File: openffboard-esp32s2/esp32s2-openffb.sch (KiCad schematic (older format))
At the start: 31 parts, among them J2 Debug, J3 CAN_Connector, J4 Motor Driver, SW1 SW_Push, SW2 SW_Push, U1 AMS1117-3.3, U3 TJA1051T-3, U5 ESP32-S2-SOLO

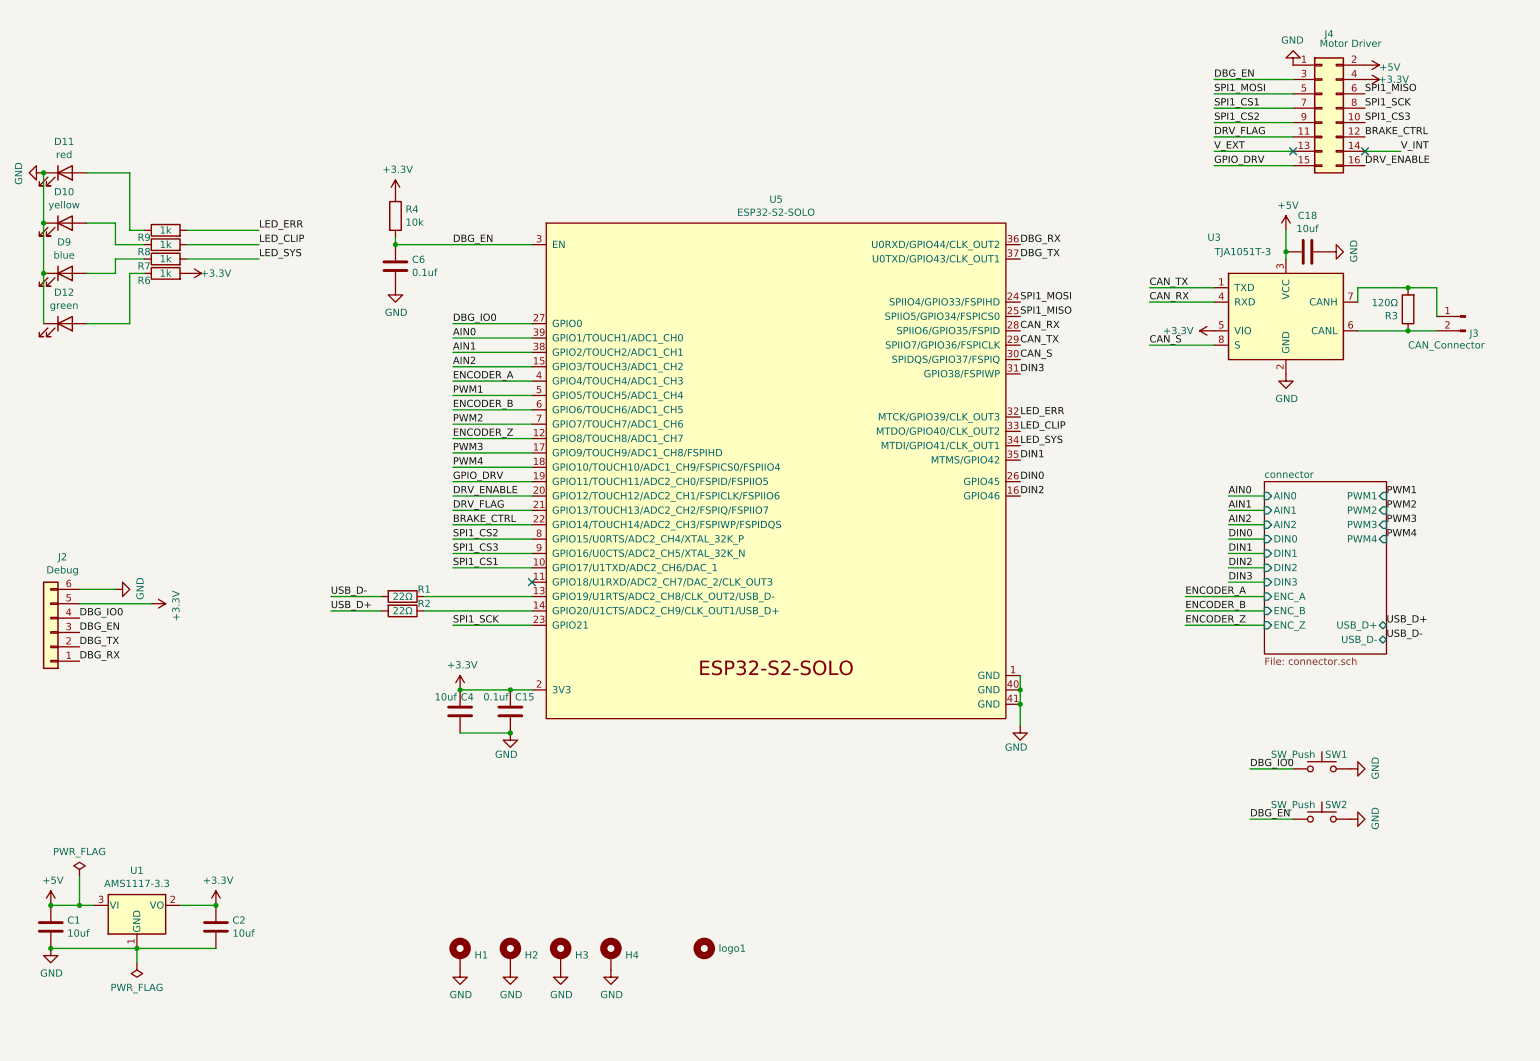
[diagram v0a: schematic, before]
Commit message: v1.1
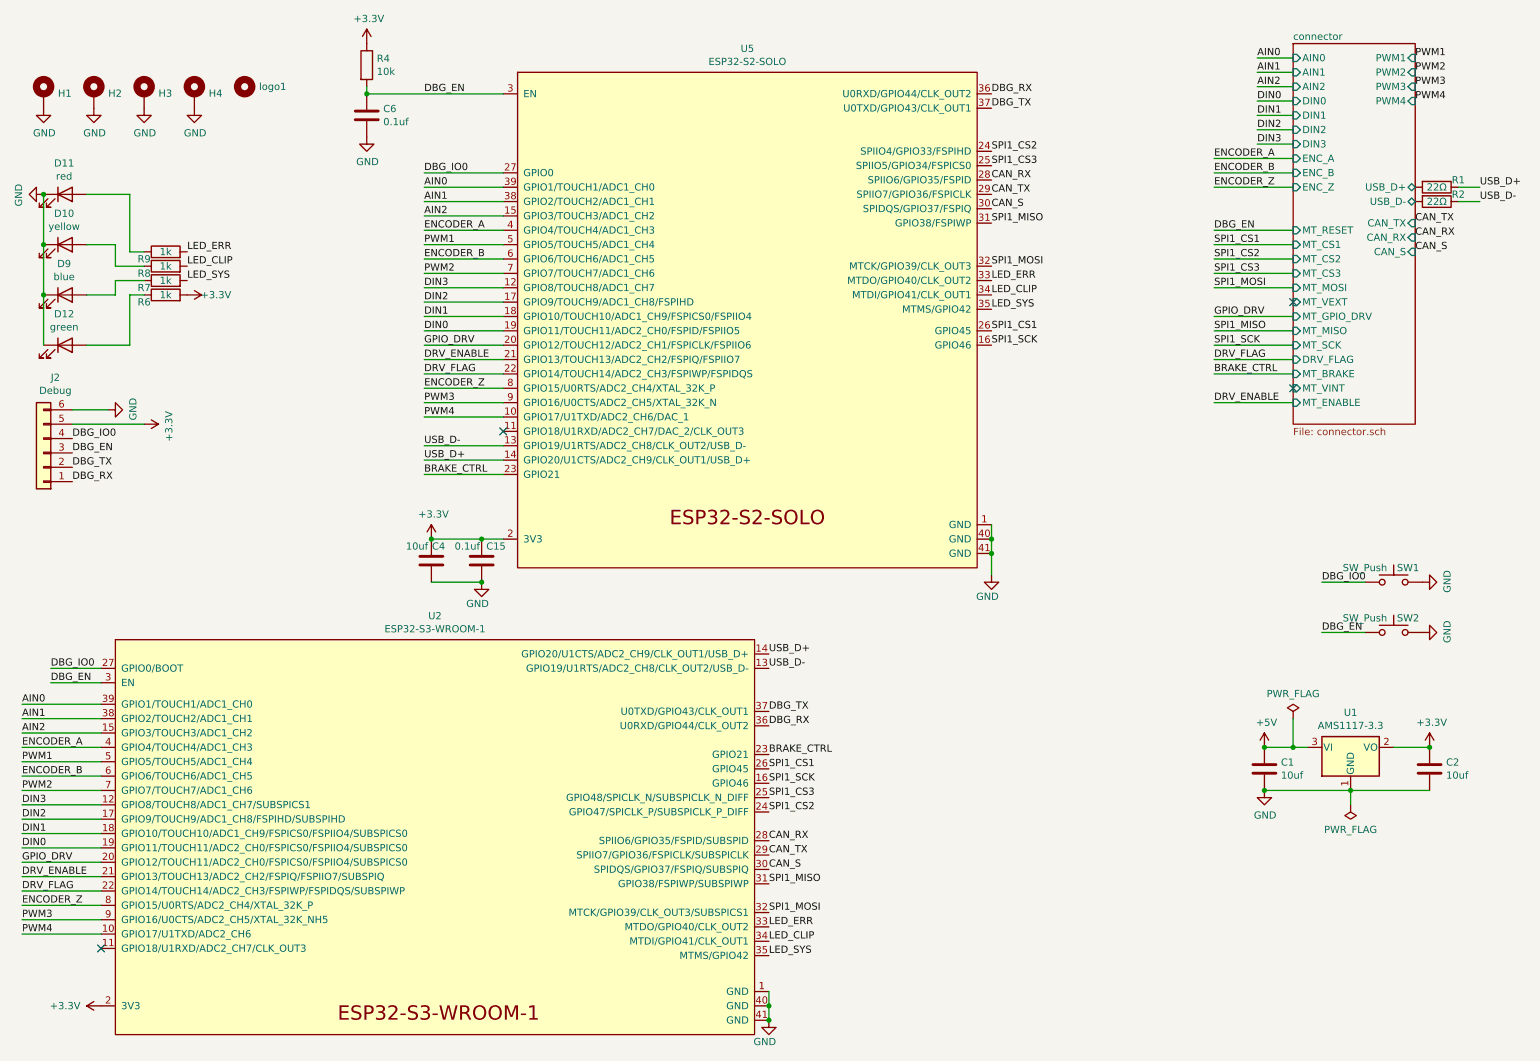
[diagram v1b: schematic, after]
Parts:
- removed C18: 10uf, Capacitor_SMD:C_0603_1608Metric, symbol Device:C
- removed J3: CAN_Connector, Connector_PinHeader_2.54mm:PinHeader_1x02_P2.54mm_Vertical, symbol Connector:Conn_01x02_Male
- removed J4: Motor Driver, Connector_PinHeader_2.54mm:PinHeader_2x08_P2.54mm_Vertical, symbol Connector_Generic:Conn_02x08_Odd_Even
- removed R3: 120Ω, Resistor_SMD:R_0603_1608Metric, symbol Device:R
- removed U3: TJA1051T-3, Package_SO:SOIC-8_3.9x4.9mm_P1.27mm, symbol Interface_CAN_LIN:TJA1051T-3
- added U2: ESP32-S3-WROOM-1, Espressif:ESP32-S3-WROOM-1, symbol Espressif:ESP32-S3-WROOM-1
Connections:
- net +3V3: now also U2.2 (3V3)
- net AIN0: now also U2.39 (GPIO1/TOUCH1/ADC1_CH0)
- net AIN1: now also U2.38 (GPIO2/TOUCH2/ADC1_CH1)
- net AIN2: now also U2.15 (GPIO3/TOUCH3/ADC1_CH2)
- net BRAKE_CTRL: now also U5.23 (GPIO21), U2.23 (GPIO21); no longer U5.22 (GPIO14/TOUCH14/ADC2_CH3/FSPIWP/FSPIDQS)
- net CAN_RX: now also U2.28 (SPIIO6/GPIO35/FSPID/SUBSPID)
- net CAN_S: now also U2.30 (SPIDQS/GPIO37/FSPIQ/SUBSPIQ)
- net CAN_TX: now also U2.29 (SPIIO7/GPIO36/FSPICLK/SUBSPICLK)
- net DBG_EN: now also U2.3 (EN)
- net DBG_IO0: now also U2.27 (GPIO0/BOOT)
- net DBG_RX: now also U2.36 (U0RXD/GPIO44/CLK_OUT2)
- net DBG_TX: now also U2.37 (U0TXD/GPIO43/CLK_OUT1)
- net DIN0: now also U5.19 (GPIO11/TOUCH11/ADC2_CH0/FSPID/FSPIIO5), U2.19 (GPIO11/TOUCH11/ADC2_CH0/FSPICS0/FSPIIO4/SUBSPICS0); no longer U5.26 (GPIO45)
- net DIN1: now also U5.18 (GPIO10/TOUCH10/ADC1_CH9/FSPICS0/FSPIIO4), U2.18 (GPIO10/TOUCH10/ADC1_CH9/FSPICS0/FSPIIO4/SUBSPICS0); no longer U5.35 (MTMS/GPIO42)
- net DIN2: now also U5.17 (GPIO9/TOUCH9/ADC1_CH8/FSPIHD), U2.17 (GPIO9/TOUCH9/ADC1_CH8/FSPIHD/SUBSPIHD); no longer U5.16 (GPIO46)
- net DIN3: now also U5.12 (GPIO8/TOUCH8/ADC1_CH7), U2.12 (GPIO8/TOUCH8/ADC1_CH7/SUBSPICS1); no longer U5.31 (GPIO38/FSPIWP)
- net DRV_ENABLE: now also U5.21 (GPIO13/TOUCH13/ADC2_CH2/FSPIQ/FSPIIO7), U2.21 (GPIO13/TOUCH13/ADC2_CH2/FSPIQ/FSPIIO7/SUBSPIQ); no longer U5.20 (GPIO12/TOUCH12/ADC2_CH1/FSPICLK/FSPIIO6)
- net DRV_FLAG: now also U5.22 (GPIO14/TOUCH14/ADC2_CH3/FSPIWP/FSPIDQS), U2.22 (GPIO14/TOUCH14/ADC2_CH3/FSPIWP/FSPIDQS/SUBSPIWP); no longer U5.21 (GPIO13/TOUCH13/ADC2_CH2/FSPIQ/FSPIIO7)
- net ENCODER_A: now also U2.4 (GPIO4/TOUCH4/ADC1_CH3)
- net ENCODER_B: now also U2.6 (GPIO6/TOUCH6/ADC1_CH5)
- net ENCODER_Z: now also U5.8 (GPIO15/U0RTS/ADC2_CH4/XTAL_32K_P), U2.8 (GPIO15/U0RTS/ADC2_CH4/XTAL_32K_P); no longer U5.12 (GPIO8/TOUCH8/ADC1_CH7)
- net GND: now also U2.1 (GND), U2.40 (GND), U2.41 (GND)
- net GPIO_DRV: now also U5.20 (GPIO12/TOUCH12/ADC2_CH1/FSPICLK/FSPIIO6), U2.20 (GPIO12/TOUCH11/ADC2_CH0/FSPICS0/FSPIIO4/SUBSPICS0); no longer U5.19 (GPIO11/TOUCH11/ADC2_CH0/FSPID/FSPIIO5)
- net LED_CLIP: now also U5.34 (MTDI/GPIO41/CLK_OUT1), U2.34 (MTDI/GPIO41/CLK_OUT1); no longer U5.33 (MTDO/GPIO40/CLK_OUT2)
- net LED_ERR: now also U5.33 (MTDO/GPIO40/CLK_OUT2), U2.33 (MTDO/GPIO40/CLK_OUT2); no longer U5.32 (MTCK/GPIO39/CLK_OUT3)
- net LED_SYS: now also U5.35 (MTMS/GPIO42), U2.35 (MTMS/GPIO42); no longer U5.34 (MTDI/GPIO41/CLK_OUT1)
- net PWM1: now also U2.5 (GPIO5/TOUCH5/ADC1_CH4)
- net PWM2: now also U2.7 (GPIO7/TOUCH7/ADC1_CH6)
- net PWM3: now also U5.9 (GPIO16/U0CTS/ADC2_CH5/XTAL_32K_N), U2.9 (GPIO16/U0CTS/ADC2_CH5/XTAL_32K_NH5); no longer U5.17 (GPIO9/TOUCH9/ADC1_CH8/FSPIHD)
- net PWM4: now also U5.10 (GPIO17/U1TXD/ADC2_CH6/DAC_1), U2.10 (GPIO17/U1TXD/ADC2_CH6); no longer U5.18 (GPIO10/TOUCH10/ADC1_CH9/FSPICS0/FSPIIO4)
- net SPI1_CS1: now also U5.26 (GPIO45), U2.26 (GPIO45); no longer U5.10 (GPIO17/U1TXD/ADC2_CH6/DAC_1)
- net SPI1_CS2: now also U5.24 (SPIIO4/GPIO33/FSPIHD), U2.24 (GPIO47/SPICLK_P/SUBSPICLK_P_DIFF); no longer U5.8 (GPIO15/U0RTS/ADC2_CH4/XTAL_32K_P)
- net SPI1_CS3: now also U5.25 (SPIIO5/GPIO34/FSPICS0), U2.25 (GPIO48/SPICLK_N/SUBSPICLK_N_DIFF); no longer U5.9 (GPIO16/U0CTS/ADC2_CH5/XTAL_32K_N)
- net SPI1_MISO: now also U5.31 (GPIO38/FSPIWP), U2.31 (GPIO38/FSPIWP/SUBSPIWP); no longer U5.25 (SPIIO5/GPIO34/FSPICS0)
- net SPI1_MOSI: now also U5.32 (MTCK/GPIO39/CLK_OUT3), U2.32 (MTCK/GPIO39/CLK_OUT3/SUBSPICS1); no longer U5.24 (SPIIO4/GPIO33/FSPIHD)
- net SPI1_SCK: now also U5.16 (GPIO46), U2.16 (GPIO46); no longer U5.23 (GPIO21)
- net USB_D+: now also R1.1, U5.14 (GPIO20/U1CTS/ADC2_CH9/CLK_OUT1/USB_D+), U2.14 (GPIO20/U1CTS/ADC2_CH9/CLK_OUT1/USB_D+); no longer R2.2
- net USB_D-: now also R2.1, U5.13 (GPIO19/U1RTS/ADC2_CH8/CLK_OUT2/USB_D-), U2.13 (GPIO19/U1RTS/ADC2_CH8/CLK_OUT2/USB_D-); no longer R1.2
- new net connector/USB_D+: R1.2
- new net connector/USB_D-: R2.2
- no-connect marks 3 -> 4
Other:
- moved on the sheet: C1, C15, C2, C4, C6, D10, D11, D12, D9, H1, H2, H3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
